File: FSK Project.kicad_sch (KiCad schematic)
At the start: 57 parts, among them J1 DATA IN, J2 TX_PAIR, J3 RX_PAIR, J4 DATA_OUT, Q1 2N3904, Q2 2N3904, SW1 MAN, U1 MC14046BCP, U2 LM393, U3 MC14046BCP

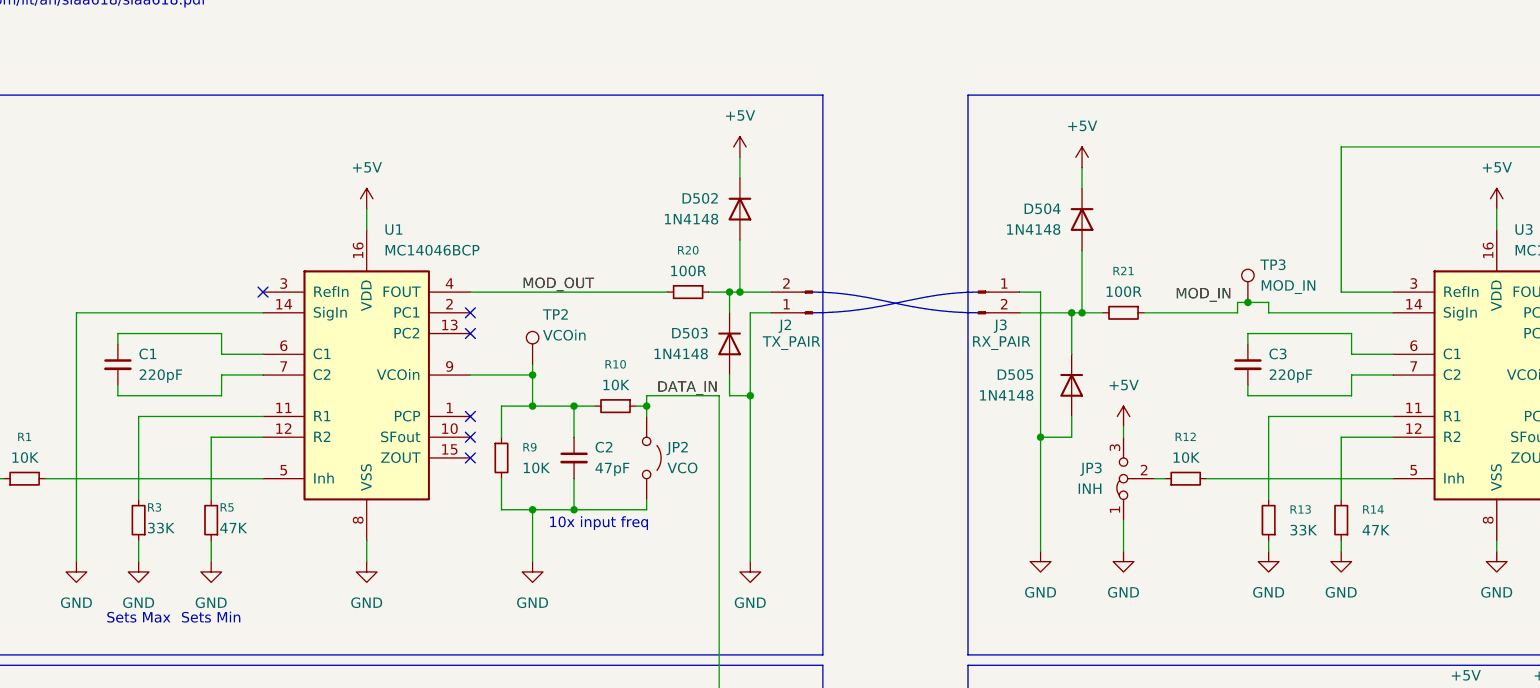
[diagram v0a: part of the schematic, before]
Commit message: fix some issues i made in the design oops
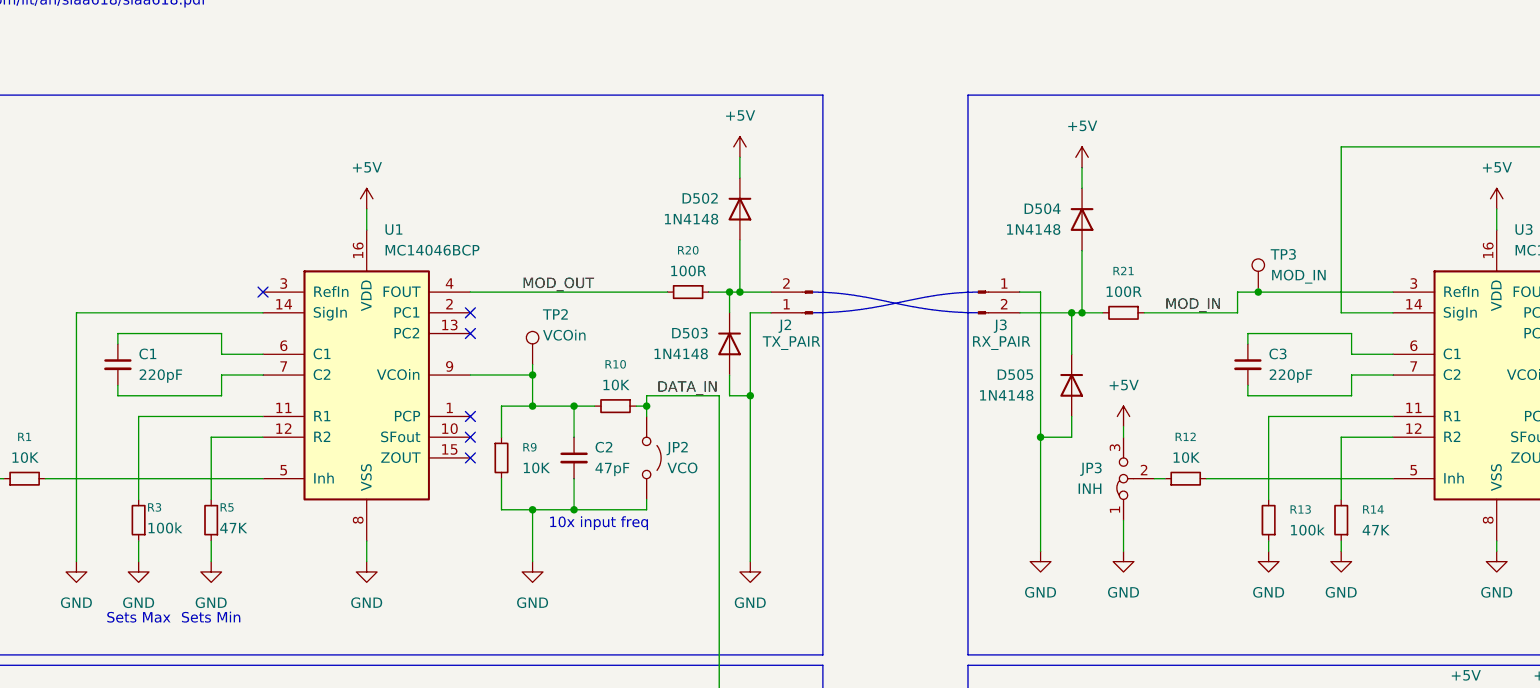
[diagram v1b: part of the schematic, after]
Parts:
- R13, R3: value 33K -> 100k
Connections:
- net MOD_IN: now also R21.1, TP3.1, U3.3 (RefIn)
- net at U3.4 (FOUT): now also U3.14 (SigIn); no longer U3.3 (RefIn)
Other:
- moved on the sheet: TP3
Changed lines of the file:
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@@
 	)
 	(junction
-		(at 181.61 54.61)
+		(at 237.49 109.22)
 		(diameter 0)
 		(color 0 0 0 0)
 	)
 	(junction
-		(at 237.49 109.22)
+		(at 99.06 67.31)
 		(diameter 0)
 		(color 0 0 0 0)
 	)
 	(junction
-		(at 99.06 67.31)
+		(at 182.88 53.34)
 		(diameter 0)
 		(color 0 0 0 0)
@@
 	(wire
 		(pts
-			(xy 184.15 54.61) (xy 184.15 55.88)
-		)
-		(stroke
-			(width 0)
-			(type default)
-		)
-	)
-	(wire
-		(pts
 			(xy 90.17 76.2) (xy 90.17 80.01)
 		)
@@
 	(wire
 		(pts
-			(xy 199.39 53.34) (xy 193.04 53.34)
-		)
-		(stroke
-			(width 0)
-			(type default)
-		)
-	)
-	(wire
-		(pts
 			(xy 118.11 66.04) (xy 120.65 66.04)
 		)
@@
 	(wire
 		(pts
-			(xy 193.04 53.34) (xy 193.04 35.56)
-		)
-		(stroke
-			(width 0)
-			(type default)
-		)
-	)
-	(wire
-		(pts
 			(xy 218.44 111.76) (xy 218.44 114.3)
 		)
@@
 	(wire
 		(pts
+			(xy 193.04 55.88) (xy 199.39 55.88)
+		)
+		(stroke
+			(width 0)
+			(type default)
+		)
+	)
+	(wire
+		(pts
 			(xy 176.53 76.2) (xy 199.39 76.2)
 		)
@@
 	(wire
 		(pts
-			(xy 180.34 54.61) (xy 181.61 54.61)
+			(xy 180.34 53.34) (xy 182.88 53.34)
 		)
 		(stroke
@@
 	(wire
 		(pts
-			(xy 180.34 54.61) (xy 180.34 55.88)
+			(xy 180.34 53.34) (xy 180.34 55.88)
 		)
 		(stroke
@@
 	(wire
 		(pts
-			(xy 181.61 54.61) (xy 184.15 54.61)
-		)
-		(stroke
-			(width 0)
-			(type default)
-		)
-	)
-	(wire
-		(pts
 			(xy 83.82 129.54) (xy 83.82 149.86)
 		)
@@
 	(wire
 		(pts
+			(xy 193.04 35.56) (xy 193.04 55.88)
+		)
+		(stroke
+			(width 0)
+			(type default)
+		)
+	)
+	(wire
+		(pts
 			(xy 267.97 66.04) (xy 267.97 73.66)
 		)
@@
 	(wire
 		(pts
+			(xy 182.88 53.34) (xy 199.39 53.34)
+		)
+		(stroke
+			(width 0)
+			(type default)
+		)
+	)
+	(wire
+		(pts
 			(xy 160.02 68.58) (xy 160.02 71.12)
 		)
@@
 	(wire
 		(pts
-			(xy 184.15 55.88) (xy 199.39 55.88)
-		)
-		(stroke
-			(width 0)
-			(type default)
-		)
-	)
-	(wire
-		(pts
 			(xy 257.81 109.22) (xy 257.81 118.11)
 		)
@@
 	)
 	(label "MOD_IN"
-		(at 172.72 54.61 0)
+		(at 171.45 55.88 0)
 		(effects
 			(font
@@
 			)
 		)
-		(property "Value" "33K"
+		(property "Value" "100k"
 			(at 186.69 82.5499 0)
 			(show_name no)
@@
 			)
 		)
-		(property "Value" "33K"
+		(property "Value" "100k"
 			(at 46.736 82.296 0)
 			(show_name no)
@@
 	(symbol
 		(lib_id "Connector:TestPoint")
-		(at 181.61 54.61 0)
+		(at 182.88 53.34 0)
 		(unit 1)
 		(body_style 1)
@@
 		(dnp no)
 		(property "Reference" "TP3"
-			(at 183.134 50.038 0)
+			(at 184.404 48.768 0)
 			(show_name no)
 			(do_not_autoplace no)
@@
 		)
 		(property "Value" "MOD_IN"
-			(at 183.134 52.578 0)
+			(at 184.404 51.308 0)
 			(show_name no)
 			(do_not_autoplace no)
@@
 		)
 		(property "Footprint" "TestPoint:TestPoint_Loop_D2.54mm_Drill1.5mm_Beaded"
-			(at 186.69 54.61 0)
+			(at 187.96 53.34 0)
 			(hide yes)
 			(show_name no)
@@
 		)
 		(property "Datasheet" ""
-			(at 186.69 54.61 0)
+			(at 187.96 53.34 0)
 			(hide yes)
 			(show_name no)
@@
 		)
 		(property "Description" "test point"
-			(at 181.61 54.61 0)
+			(at 182.88 53.34 0)
 			(hide yes)
 			(show_name no)
